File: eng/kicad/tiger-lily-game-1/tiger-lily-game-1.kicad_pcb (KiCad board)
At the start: 2 copper layers, 99.1 x 99.1 mm, 17 parts, among them J1 Conn_01x06_Male, SW1 SW_PWR, SW2 SW_RESET, SW3 SW_P1, SW4 SW_PLAY, SW5 SW_P2, U1 PIC16F15323-IP

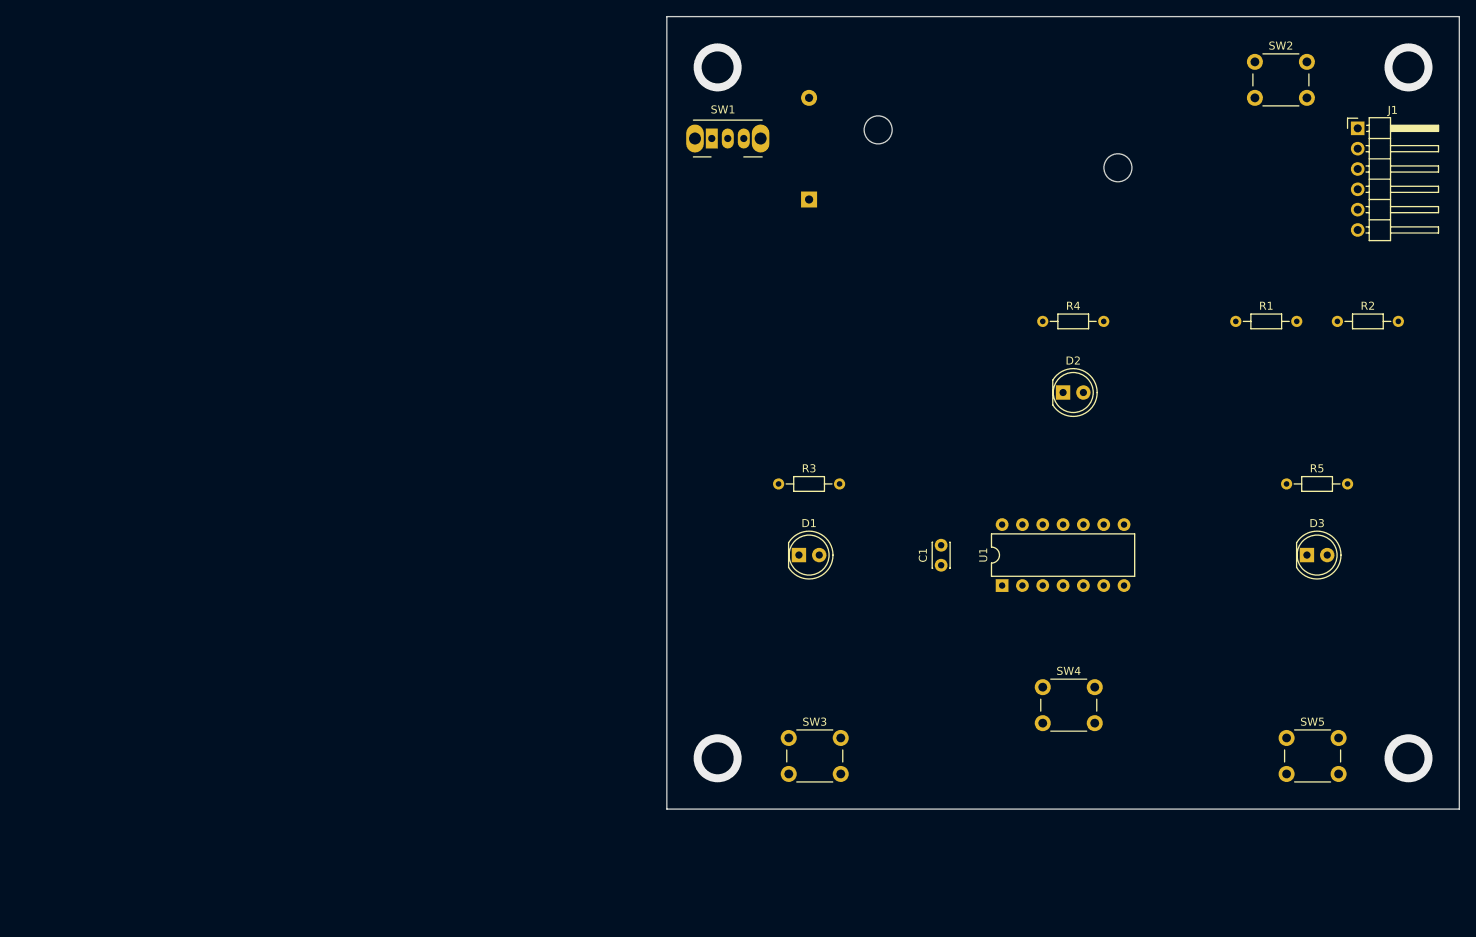
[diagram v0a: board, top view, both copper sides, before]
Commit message: Schematic and PCB design (WIP). Firmware (WIP). Checked in for backup.
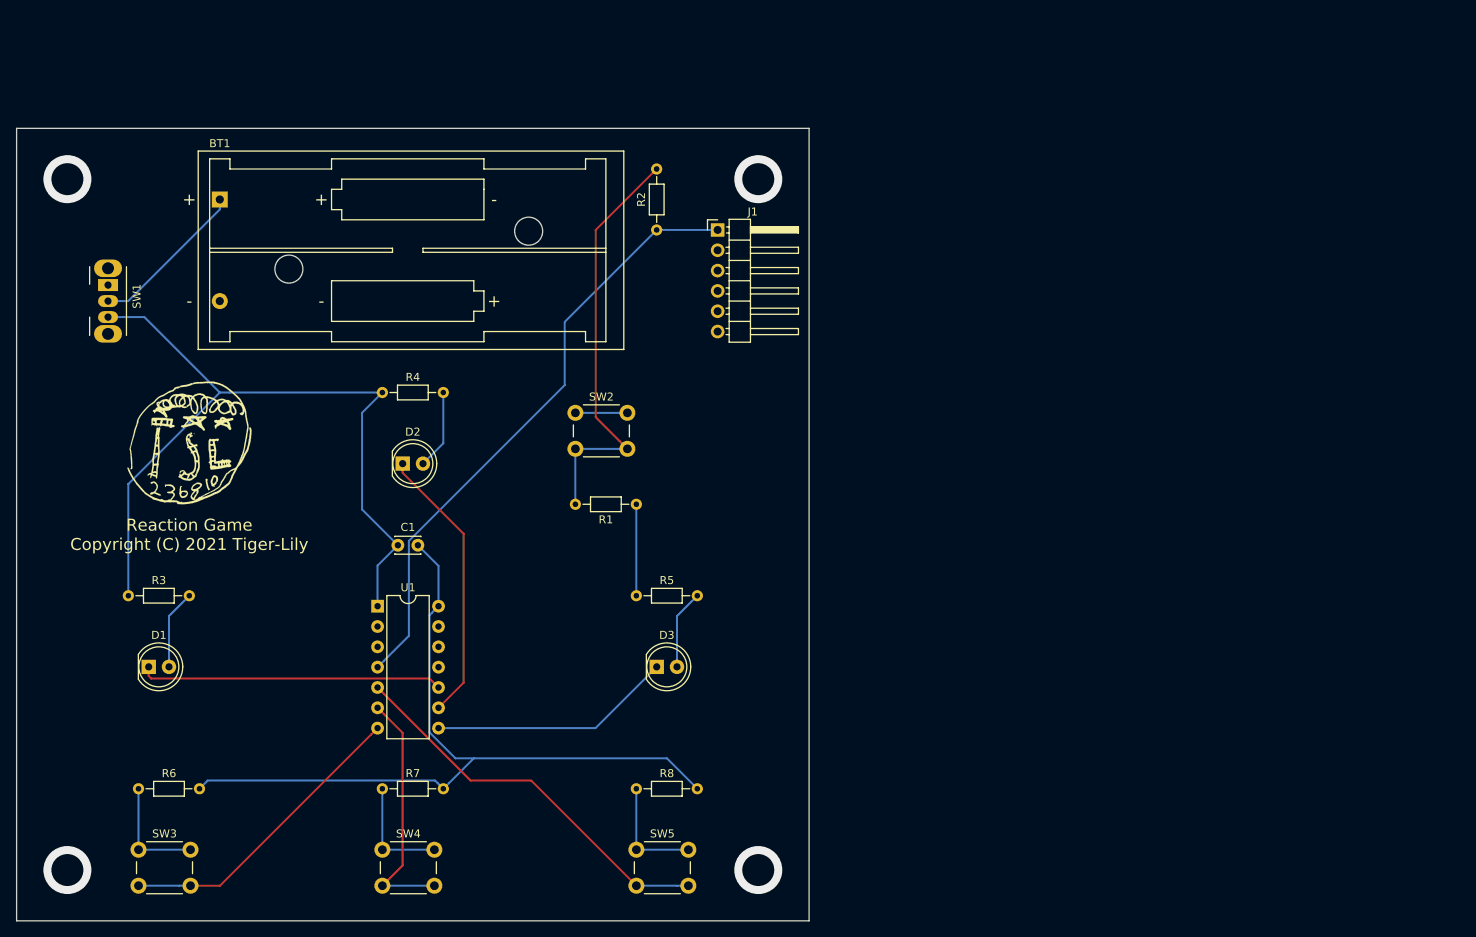
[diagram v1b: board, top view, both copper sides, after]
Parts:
- added G***: LOGO, tiger-lily-logo:tiger-lily-logo-160, F.Cu at (111.8, 91.4)
- added R6: 330R, Resistor_THT:R_Axial_DIN0204_L3.6mm_D1.6mm_P7.62mm_Horizontal, F.Cu at (105.4, 134.6)
- added R7: 330R, Resistor_THT:R_Axial_DIN0204_L3.6mm_D1.6mm_P7.62mm_Horizontal, F.Cu at (135.9, 134.6)
- added R8: 330R, Resistor_THT:R_Axial_DIN0204_L3.6mm_D1.6mm_P7.62mm_Horizontal, F.Cu at (167.6, 134.6)
- BT1: moved to F.Cu
- moved SW2 95.6 mm to (160.0, 87.6)
- moved R2 85.9 mm to (170.2, 64.8), turned to 90 degrees
- moved SW4 85.0 mm to (135.9, 142.2)
- moved R4 83.0 mm to (135.9, 85.1)
- moved D2 83.0 mm to (138.4, 94.0)
- moved D1 82.5 mm to (106.7, 119.4)
- moved D3 82.5 mm to (170.2, 119.4)
- moved R5 82.5 mm to (167.6, 110.5)
- moved SW3 82.5 mm to (105.4, 142.2)
- moved SW5 82.5 mm to (167.6, 142.2)
- moved R3 82.5 mm to (104.1, 110.5)
- moved J1 81.0 mm to (177.8, 64.8)
- moved R1 78.3 mm to (167.6, 99.1), turned to 180 degrees
- moved U1 78.1 mm to (135.3, 111.8), turned to 0 degrees
- moved SW1 77.7 mm to (101.6, 71.7), turned to 270 degrees
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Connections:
- D1 pad 1: (no net) -> /LED_P1
- D1 pad 2: (no net) -> Net-(D1-Pad2)
- D2 pad 1: (no net) -> /LED_GO
- D2 pad 2: (no net) -> Net-(D2-Pad2)
- D3 pad 1: (no net) -> /LED_P2
- D3 pad 2: (no net) -> Net-(D3-Pad2)
- J1 pad 1: (no net) -> /MCU_VPP
- J1 pad 4: (no net) -> /MCU_ICSPXXX
- J1 pad 5: (no net) -> /MCU_ICSPYYY
- J1 pad 6: (no net) -> Net-(J1-Pad6)
- R1 pad 1: (no net) -> /MCU_PWR
- R1 pad 2: (no net) -> Net-(R1-Pad2)
- R2 pad 1: (no net) -> /MCU_VPP
- R2 pad 2: (no net) -> Net-(R1-Pad2)
- R3 pad 1: (no net) -> /MCU_PWR
- R3 pad 2: (no net) -> Net-(D1-Pad2)
- R4 pad 1: (no net) -> /MCU_PWR
- R4 pad 2: (no net) -> Net-(D2-Pad2)
- R5 pad 1: (no net) -> /MCU_PWR
- R5 pad 2: (no net) -> Net-(D3-Pad2)
- SW2 pad 1: Net-(SW2-Pad1) -> /MCU_GND
- SW2 pad 2: Net-(SW2-Pad2) -> Net-(R1-Pad2)
- SW3 pad 2: Net-(SW3-Pad2) -> /SW_P1
- SW4 pad 2: Net-(SW4-Pad2) -> /SW_GO
- SW5 pad 2: Net-(SW5-Pad2) -> /SW_P2
- U1 pad 10: (no net) -> /LED_P1
- U1 pad 11: (no net) -> Net-(U1-Pad11)
- U1 pad 12: (no net) -> /MCU_ICSPYYY
- U1 pad 13: (no net) -> /MCU_ICSPXXX
- U1 pad 2: (no net) -> Net-(U1-Pad2)
- U1 pad 3: (no net) -> Net-(U1-Pad3)
- U1 pad 4: (no net) -> /MCU_VPP
- U1 pad 5: (no net) -> /SW_P2
- U1 pad 6: (no net) -> /SW_GO
- U1 pad 7: (no net) -> /SW_P1
- U1 pad 8: (no net) -> /LED_P2
- U1 pad 9: (no net) -> /LED_GO
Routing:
- net /MCU_PWR: track 0.00 -> 110.4 mm
- net /MCU_GND: track 0.00 -> 104.5 mm
- net /MCU_VPP: track 0.00 -> 76.7 mm
- net Net-(R1-Pad2): track 0.00 -> 53.2 mm
- net /SW_P2: track 0.00 -> 49.1 mm
- net /SW_P1: track 0.00 -> 38.0 mm
- net /LED_P1: track 0.00 -> 38.0 mm
- net /LED_GO: track 0.00 -> 35.0 mm
- net /SW_GO: track 0.00 -> 31.1 mm
- net /LED_P2: track 0.00 -> 30.4 mm
- net Net-(BT1-Pad1): track 0.00 -> 20.0 mm
- net Net-(R8-Pad1): track 0.00 -> 14.1 mm
- net Net-(R7-Pad1): track 0.00 -> 14.1 mm
- net Net-(R6-Pad1): track 0.00 -> 14.1 mm
- net Net-(D1-Pad2): track 0.00 -> 9.94 mm
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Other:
- board text added: "Reaction Game Copyright (C) 2021 Tiger-Lily"
